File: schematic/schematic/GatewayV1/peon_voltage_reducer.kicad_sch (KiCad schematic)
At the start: 14 parts, among them Q1 BSS138, Q2 SFH3201, U2 LM358

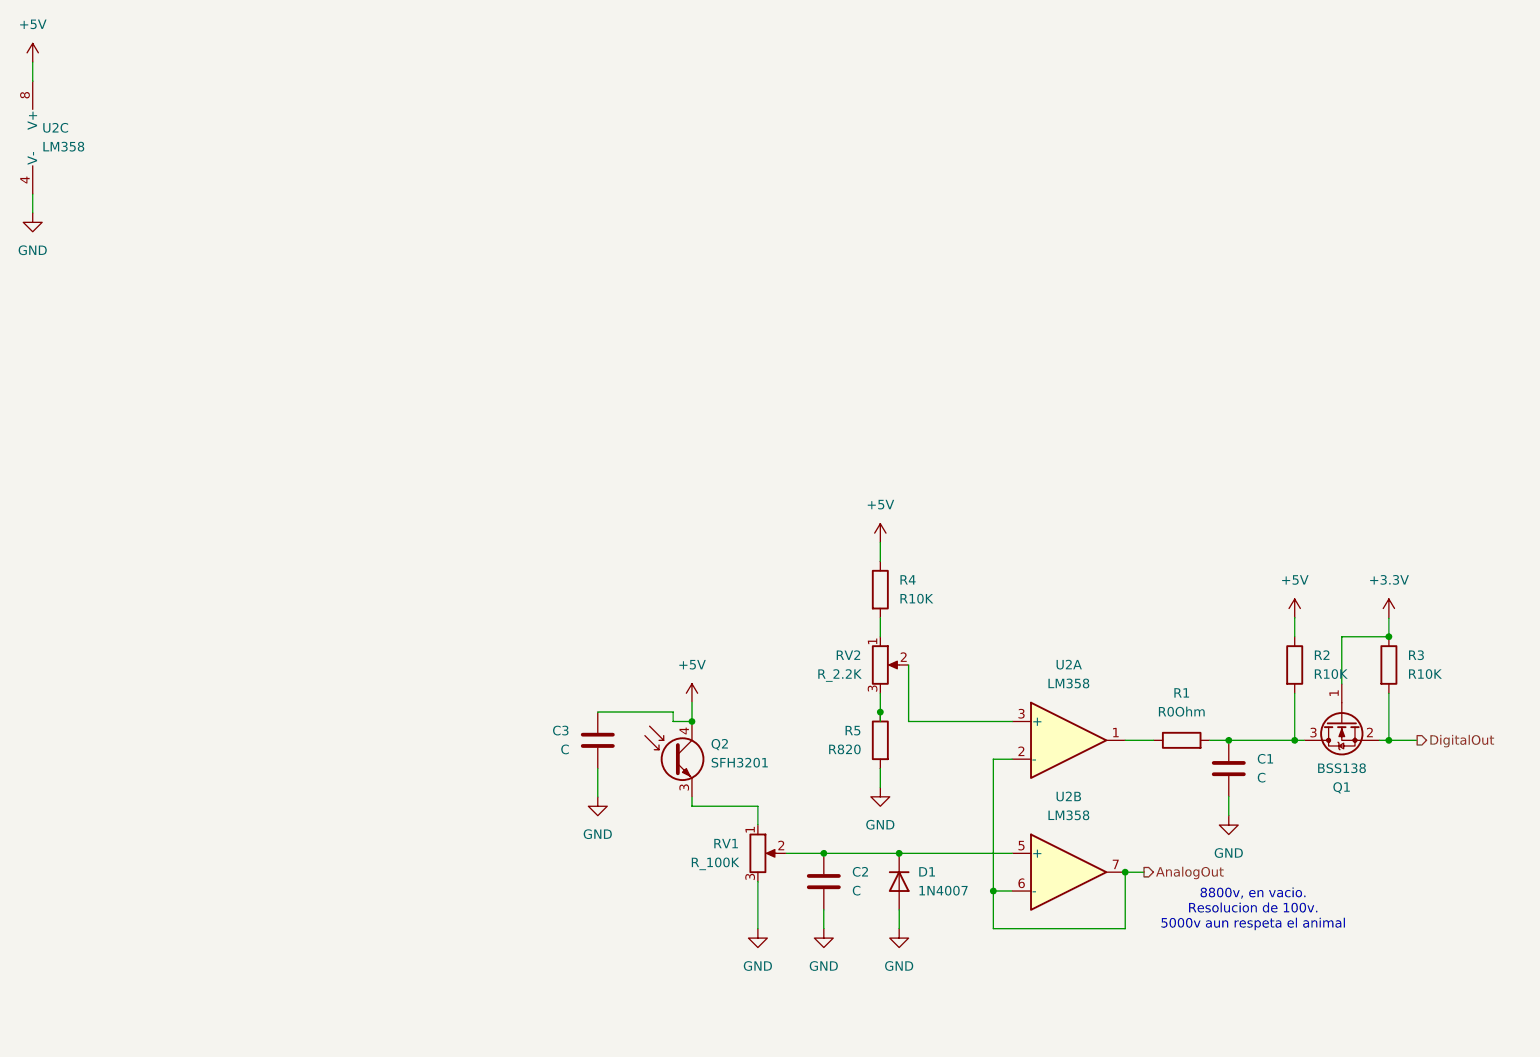
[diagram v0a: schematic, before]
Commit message: Feat: Updated components
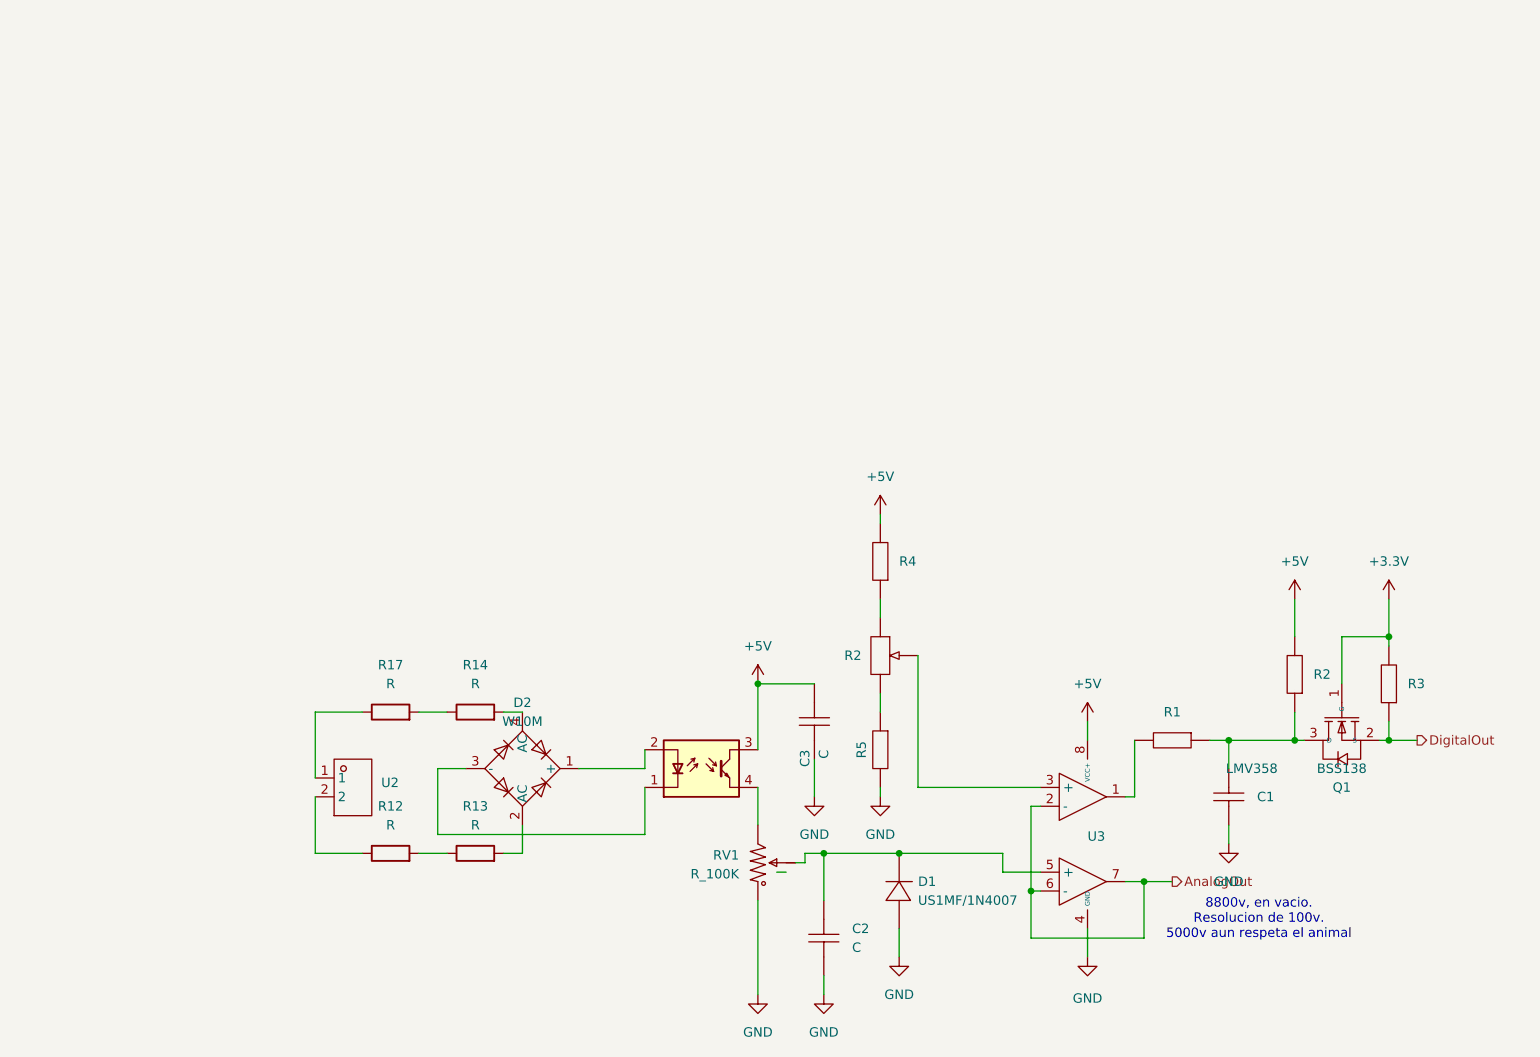
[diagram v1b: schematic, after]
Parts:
- removed Q2: SFH3201, OptoDevice:Osram_SFH9x0x, symbol Sensor_Optical:SFH3201
- removed U2: LM358, symbol Amplifier_Operational:LM358
- added D2: W10M, easyEDA:DIO-BG-TH_W10M, symbol easyEDA:W10M
- added R12, R13, R14, R17: R, symbol Device:R
- added U2: ~, easyEDA:CONN-TH_KF88SA-16.0-2P, symbol easyEDA:KF88SA-16.0-2P
- added U3: LMV358, easyEDA:SOIC-8_L4.9-W3.9-P1.27-LS6.0-BL, symbol easyEDA:LMV358IDR
- added U7: ~, ibSolutions:PEON_IR_INSULATION_v1, symbol ibSolutions:Peon_IR_High_Voltage_Insulation
- C1: value C -> 100nF; footprint (none) -> easyEDA:C1206; symbol Device:C -> easyEDA:CL31B104KBCNNNC; LCSC Part Name (none) -> 100nF ±10% 50V; Manufacturer (none) -> SAMSUNG(三星); Manufacturer Part (none) -> CL31B104KBCNNNC; Supplier (none) -> LCSC; Supplier Part (none) -> C24497
- C2, C3: footprint (none) -> easyEDA:C1206; symbol Device:C -> easyEDA:CC1206KRX7R9BB104; LCSC Part Name (none) -> 100nF ±10% 50V; Manufacturer (none) -> YAGEO(国巨); Manufacturer Part (none) -> CC1206KRX7R9BB104; Supplier (none) -> LCSC; Supplier Part (none) -> C82601
- D1: value 1N4007 -> US1MF/1N4007; footprint Diode_THT:D_DO-41_SOD81_P10.16mm_Horizontal -> easyEDA:SMAF_L3.5-W2.6-LS4.7-RD; symbol Diode:1N4007 -> easyEDA:US1MF_C64877; LCSC Part Name (none) -> 电压:1kV 电流:1A; Manufacturer (none) -> MDD(辰达半导体); Manufacturer Part (none) -> US1MF; Supplier (none) -> LCSC; Supplier Part (none) -> C64877
- Q1: footprint Package_TO_SOT_SMD:SOT-23 -> easyEDA:SOT-23-3_L2.9-W1.6-P1.90-LS2.8-BR; symbol Transistor_FET:BSS138 -> easyEDA:BSS138-7-F; LCSC Part Name (none) -> 1个N沟道 耐压:50V 电流:200mA; Manufacturer (none) -> DIODES(美台); Manufacturer Part (none) -> BSS138-7-F; Supplier (none) -> LCSC; Supplier Part (none) -> C40912
- R1: value R0Ohm -> 0Ω; footprint (none) -> easyEDA:R1206; symbol Device:R -> easyEDA:1206 J000T5E; LCSC Part Name (none) -> 0Ω ±5% 250mW 厚膜电阻; Manufacturer (none) -> UNI-ROYAL(厚声); Manufacturer Part (none) -> 1206W4J0000T5E; Supplier (none) -> LCSC; Supplier Part (none) -> C19290
- R2, R3, R4: value R10K -> 10kΩ; footprint (none) -> easyEDA:R1206; symbol Device:R -> easyEDA:1206W4F1002T5E; LCSC Part Name (none) -> 10kΩ ±1% 250mW 厚膜电阻; Manufacturer (none) -> UNI-ROYAL(厚声); Manufacturer Part (none) -> 1206W4F1002T5E; Supplier (none) -> LCSC; Supplier Part (none) -> C17902
- R2: renamed from RV2; value R_2.2K -> 2kΩ/2.2K; footprint (none) -> easyEDA:RES-ADJ-TH_3P-L7.1-W6.9-P2.50-L_3362P; symbol Device:R_Potentiometer -> easyEDA:3362P-1-202_C118929; LCSC Part Name (none) -> 2kΩ ±10%; Manufacturer (none) -> BOCHEN(博晨); Manufacturer Part (none) -> 3362P-1-202; Supplier (none) -> LCSC; Supplier Part (none) -> C118929
- R5: value R820 -> 820Ω; footprint (none) -> easyEDA:R1206; symbol Device:R -> easyEDA:1206W4F8200T5E; LCSC Part Name (none) -> 820Ω ±1% 250mW 厚膜电阻; Manufacturer (none) -> UNI-ROYAL(厚声); Manufacturer Part (none) -> 1206W4F8200T5E; Supplier (none) -> LCSC; Supplier Part (none) -> C17984
- RV1: footprint (none) -> easyEDA:RES-ADJ-TH_3362P; symbol Device:R_Potentiometer -> easyEDA:3362P-1-104_C118966; LCSC Part Name (none) -> 100kΩ ±10%; Manufacturer (none) -> BOCHEN(博晨); Manufacturer Part (none) -> 3362P-1-104; Supplier (none) -> LCSC; Supplier Part (none) -> C118966
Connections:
- net +3.3V: now also R3.2; no longer R3.1
- net +5V: now also R2.2, R4.2, U3.8 (VCC+), U7.3; no longer R2.1, R4.1
- net AnalogOut: now also U3.2 (-), U3.6 (-), U3.7
- net DigitalOut: now also R3.1; no longer R3.2
- net GND: now also C1.1, C2.1, RV1.1, U3.4 (GND); no longer C1.2, C2.2, RV1.3
- net at D1.1 (K), RV1.2: now also C2.2, U3.5 (+); no longer C2.1
- net at R2.1: now also R4.1; no longer R4.2
- net at R1.1: now also C1.2, Q1.3 (D), R2.1
- net at R2.2: now also U3.3 (+)
- new net: R14.1, R17.2
- new net: D2.4 (AC), R14.2
- new net: RV1.3, U7.4
- new net: R12.1, U2.2
- new net: R12.2, R13.1
- new net: R17.1, U2.1
- new net: D2.3 (-), U7.1
- new net: D2.1 (+), U7.2
- new net: D2.2 (AC), R13.2
- new net: R1.2, U3.1
